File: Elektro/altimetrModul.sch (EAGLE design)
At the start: 16 parts, among them IC1 ATTINY1624-SSU, J1 SM04B-GHS-TB(LF)(SN)-

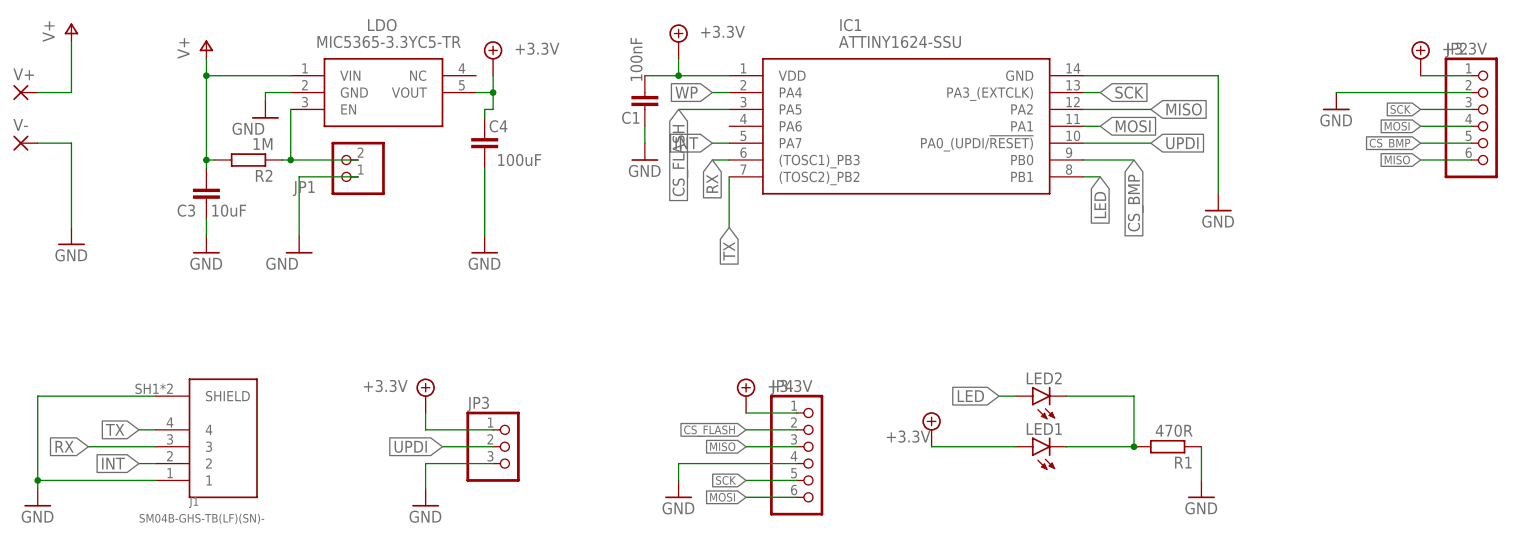
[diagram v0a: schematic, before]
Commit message: Added names
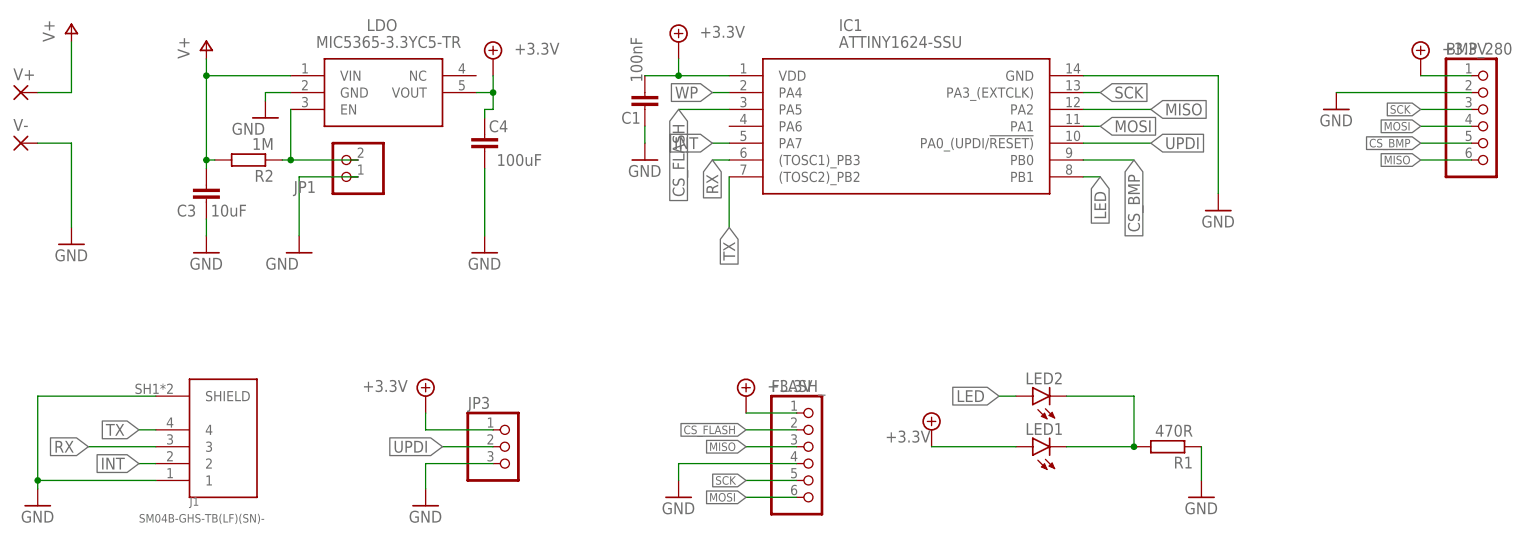
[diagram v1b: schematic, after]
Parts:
- renumbered JP2 to BMP_280, JP4 to FLASH_
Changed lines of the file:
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@@
 <part name="U$8" library="supply2" deviceset="+3.3V" device=""/>
 <part name="GND1" library="PUTRocketLab_supply" deviceset="GND" device=""/>
-<part name="JP2" library="pinhead" library_urn="urn:adsk.eagle:library:325" deviceset="PINHD-1X6" device="" package3d_urn="urn:adsk.eagle:package:22472/2"/>
-<part name="JP4" library="pinhead" library_urn="urn:adsk.eagle:library:325" deviceset="PINHD-1X6" device="" package3d_urn="urn:adsk.eagle:package:22472/2"/>
+<part name="BMP_280" library="pinhead" library_urn="urn:adsk.eagle:library:325" deviceset="PINHD-1X6" device="" package3d_urn="urn:adsk.eagle:package:22472/2"/>
+<part name="FLASH_" library="pinhead" library_urn="urn:adsk.eagle:library:325" deviceset="PINHD-1X6" device="" package3d_urn="urn:adsk.eagle:package:22472/2"/>
 <part name="U$5" library="supply2" deviceset="+3.3V" device=""/>
 <part name="U$7" library="supply2" deviceset="+3.3V" device=""/>
@@
 <attribute name="VALUE" x="-160.02" y="36.83" size="1.778" layer="96"/>
 </instance>
-<instance part="JP2" gate="A" x="60.96" y="96.52" smashed="yes" grouprefs="BMP280">
+<instance part="BMP_280" gate="A" x="60.96" y="96.52" smashed="yes" grouprefs="BMP280">
 <attribute name="NAME" x="54.61" y="107.315" size="1.778" layer="95"/>
 <attribute name="VALUE" x="54.61" y="86.36" size="1.778" layer="96"/>
 </instance>
-<instance part="JP4" gate="A" x="-40.64" y="45.72" smashed="yes" grouprefs="FLASH">
+<instance part="FLASH_" gate="A" x="-40.64" y="45.72" smashed="yes" grouprefs="FLASH">
 <attribute name="NAME" x="-46.99" y="56.515" size="1.778" layer="95"/>
 <attribute name="VALUE" x="-46.99" y="35.56" size="1.778" layer="96"/>
@@
 </segment>
 <segment>
-<pinref part="JP2" gate="A" pin="2"/>
+<pinref part="BMP_280" gate="A" pin="2"/>
 <pinref part="GND5" gate="1" pin="GND"/>
 <wire x1="38.1" y1="101.6" x2="58.42" y2="101.6" width="0.1524" layer="91" grouprefs="BMP280"/>
@@
 <pinref part="GND8" gate="1" pin="GND"/>
 <wire x1="-60.96" y1="43.18" x2="-60.96" y2="45.72" width="0.1524" layer="91" grouprefs="FLASH"/>
-<pinref part="JP4" gate="A" pin="4"/>
+<pinref part="FLASH_" gate="A" pin="4"/>
 <wire x1="-60.96" y1="45.72" x2="-43.18" y2="45.72" width="0.1524" layer="91" grouprefs="FLASH"/>
 </segment>
@@
 </segment>
 <segment>
-<pinref part="JP2" gate="A" pin="1"/>
+<pinref part="BMP_280" gate="A" pin="1"/>
 <wire x1="58.42" y1="104.14" x2="50.8" y2="104.14" width="0.1524" layer="91" grouprefs="BMP280"/>
 <pinref part="U$5" gate="G$1" pin="+3.3V"/>
 </segment>
 <segment>
-<pinref part="JP4" gate="A" pin="1"/>
+<pinref part="FLASH_" gate="A" pin="1"/>
 <wire x1="-43.18" y1="53.34" x2="-50.8" y2="53.34" width="0.1524" layer="91" grouprefs="FLASH"/>
 <pinref part="U$7" gate="G$1" pin="+3.3V"/>
@@
 <wire x1="58.42" y1="99.06" x2="50.8" y2="99.06" width="0.1524" layer="91" grouprefs="BMP280"/>
 <label x="50.8" y="99.06" size="1.27" layer="95" rot="R180" xref="yes" grouprefs="BMP280"/>
-<pinref part="JP2" gate="A" pin="3"/>
+<pinref part="BMP_280" gate="A" pin="3"/>
 </segment>
 <segment>
 <wire x1="-43.18" y1="43.18" x2="-50.8" y2="43.18" width="0.1524" layer="91" grouprefs="FLASH"/>
 <label x="-50.8" y="43.18" size="1.27" layer="95" rot="R180" xref="yes" grouprefs="FLASH"/>
-<pinref part="JP4" gate="A" pin="5"/>
+<pinref part="FLASH_" gate="A" pin="5"/>
 </segment>
 </net>
@@
 <wire x1="58.42" y1="91.44" x2="50.8" y2="91.44" width="0.1524" layer="91" grouprefs="BMP280"/>
 <label x="50.8" y="91.44" size="1.27" layer="95" rot="R180" xref="yes" grouprefs="BMP280"/>
-<pinref part="JP2" gate="A" pin="6"/>
-</segment>
-<segment>
-<pinref part="JP4" gate="A" pin="3"/>
+<pinref part="BMP_280" gate="A" pin="6"/>
+</segment>
+<segment>
+<pinref part="FLASH_" gate="A" pin="3"/>
 <wire x1="-43.18" y1="48.26" x2="-50.8" y2="48.26" width="0.1524" layer="91"/>
 <label x="-50.8" y="48.26" size="1.27" layer="95" rot="R180" xref="yes"/>
@@
 <wire x1="58.42" y1="96.52" x2="50.8" y2="96.52" width="0.1524" layer="91" grouprefs="BMP280"/>
 <label x="50.8" y="96.52" size="1.27" layer="95" rot="R180" xref="yes" grouprefs="BMP280"/>
-<pinref part="JP2" gate="A" pin="4"/>
+<pinref part="BMP_280" gate="A" pin="4"/>
 </segment>
 <segment>
 <wire x1="-43.18" y1="40.64" x2="-50.8" y2="40.64" width="0.1524" layer="91" grouprefs="FLASH"/>
 <label x="-50.8" y="40.64" size="1.27" layer="95" rot="R180" xref="yes" grouprefs="FLASH"/>
-<pinref part="JP4" gate="A" pin="6"/>
+<pinref part="FLASH_" gate="A" pin="6"/>
 </segment>
 </net>
@@
 <wire x1="58.42" y1="93.98" x2="50.8" y2="93.98" width="0.1524" layer="91" grouprefs="BMP280"/>
 <label x="50.8" y="93.98" size="1.27" layer="95" rot="R180" xref="yes" grouprefs="BMP280"/>
-<pinref part="JP2" gate="A" pin="5"/>
+<pinref part="BMP_280" gate="A" pin="5"/>
 </segment>
 </net>
@@
 <wire x1="-43.18" y1="50.8" x2="-50.8" y2="50.8" width="0.1524" layer="91" grouprefs="FLASH"/>
 <label x="-50.8" y="50.8" size="1.27" layer="95" rot="R180" xref="yes" grouprefs="FLASH"/>
-<pinref part="JP4" gate="A" pin="2"/>
-</segment>
-</net>
+<pinref part="FLASH_" gate="A" pin="2"/>
+</segment>
+</net>
